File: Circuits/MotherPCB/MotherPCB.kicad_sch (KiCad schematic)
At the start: 0 parts

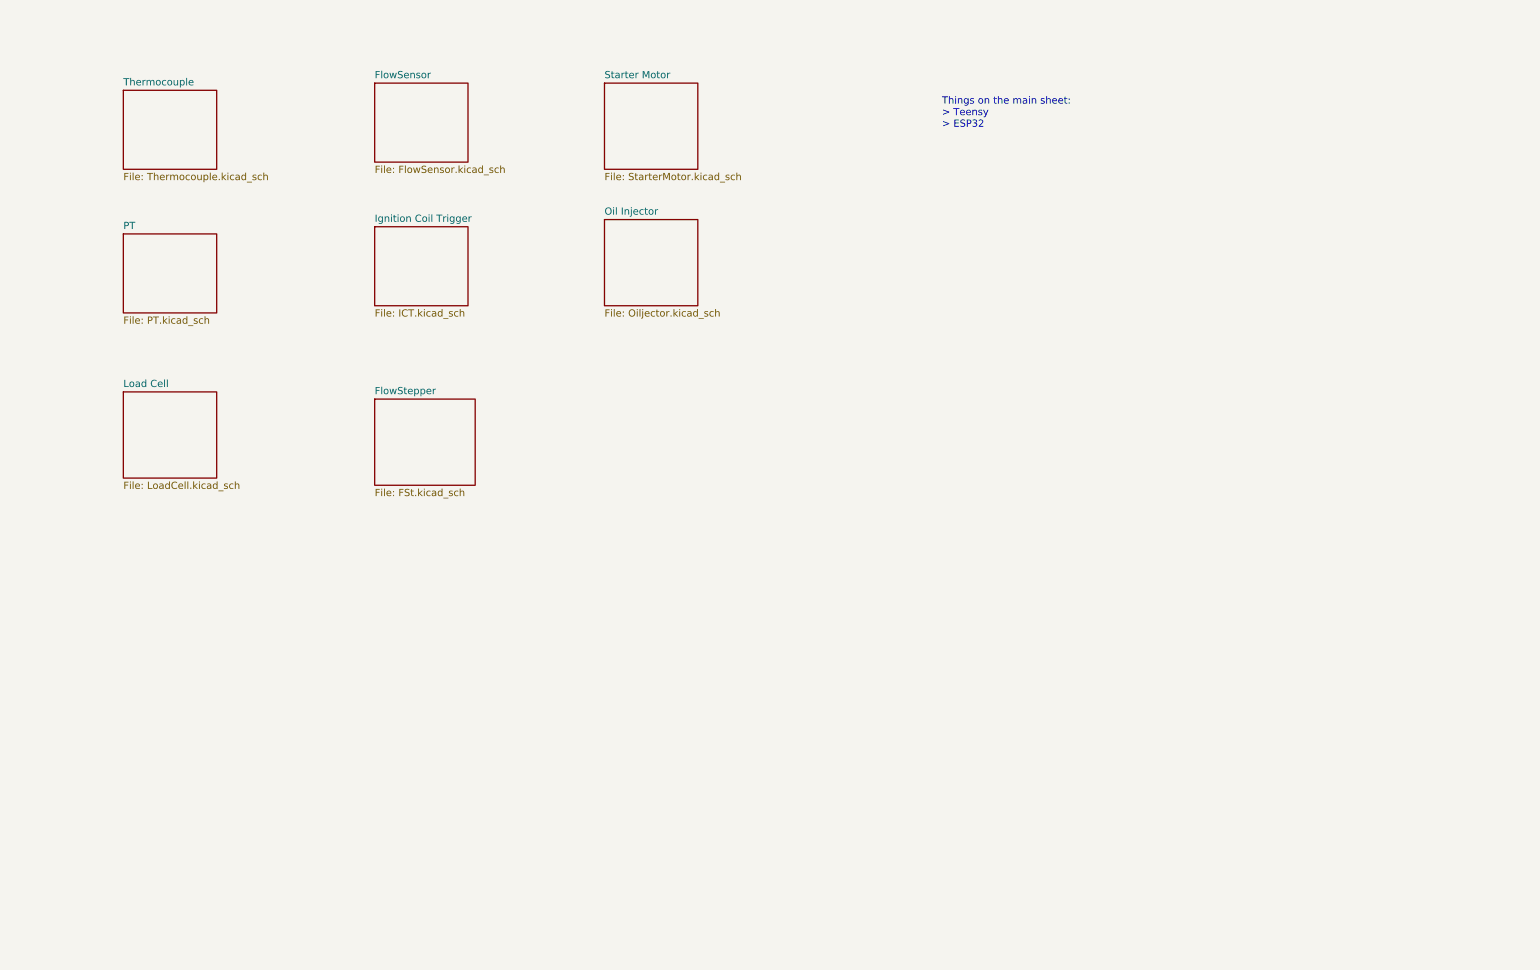
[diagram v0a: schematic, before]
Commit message: Done for the night
Finished up thermocouple differential communication and every other module apart from PTs and Oil Injector.

Good night.
oh wait
It's 4:00 am.
Good morning
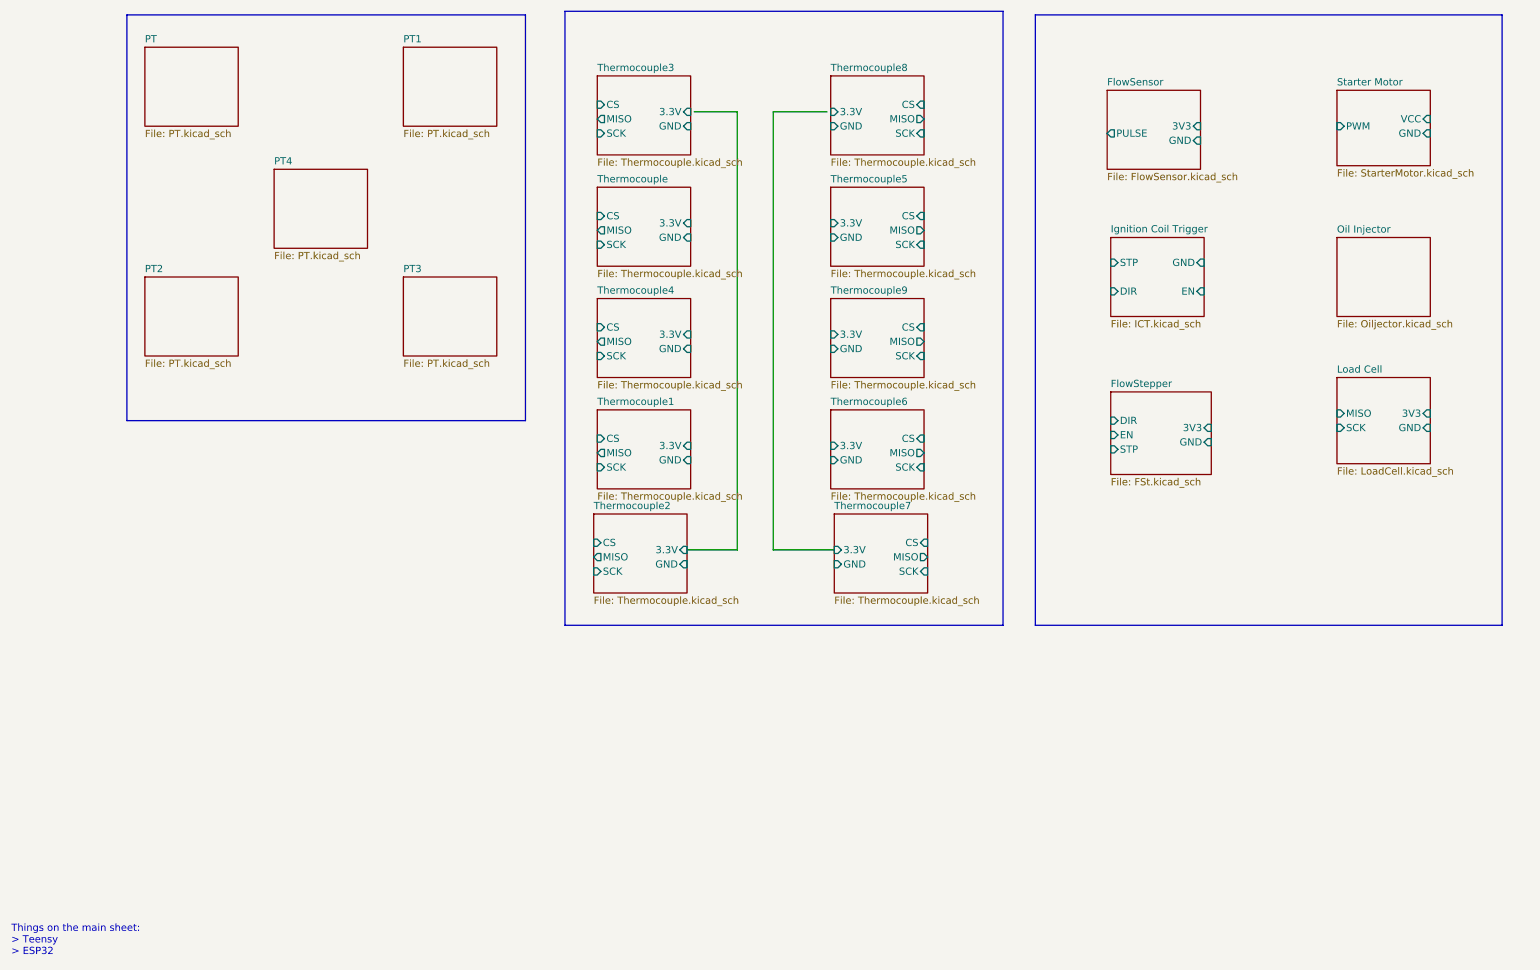
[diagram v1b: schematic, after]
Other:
- added sheet PT1 (PT.kicad_sch)
- added sheet PT2 (PT.kicad_sch)
- added sheet PT3 (PT.kicad_sch)
- added sheet PT4 (PT.kicad_sch)
- added sheet Thermocouple1 (Thermocouple.kicad_sch)
- added sheet Thermocouple2 (Thermocouple.kicad_sch)
- added sheet Thermocouple3 (Thermocouple.kicad_sch)
- added sheet Thermocouple4 (Thermocouple.kicad_sch)
- added sheet Thermocouple5 (Thermocouple.kicad_sch)
- added sheet Thermocouple6 (Thermocouple.kicad_sch)
- added sheet Thermocouple7 (Thermocouple.kicad_sch)
- added sheet Thermocouple8 (Thermocouple.kicad_sch)
- added sheet Thermocouple9 (Thermocouple.kicad_sch)
- sheet FlowSensor ports: added 3V3, GND, PULSE; removed none
- sheet FlowStepper ports: added 3V3, DIR, EN, GND, STP; removed none
- sheet Ignition Coil Trigger ports: added DIR, EN, GND, STP; removed none
- sheet Load Cell ports: added 3V3, GND, MISO, SCK; removed none
- sheet Starter Motor ports: added GND, PWM, VCC; removed none
- sheet Thermocouple ports: added 3.3V, CS, GND, MISO, SCK; removed none
- company: (none) -> Project Arka
- title: (none) -> ECU Motherboard
